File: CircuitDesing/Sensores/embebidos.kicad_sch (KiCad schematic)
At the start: 15 parts

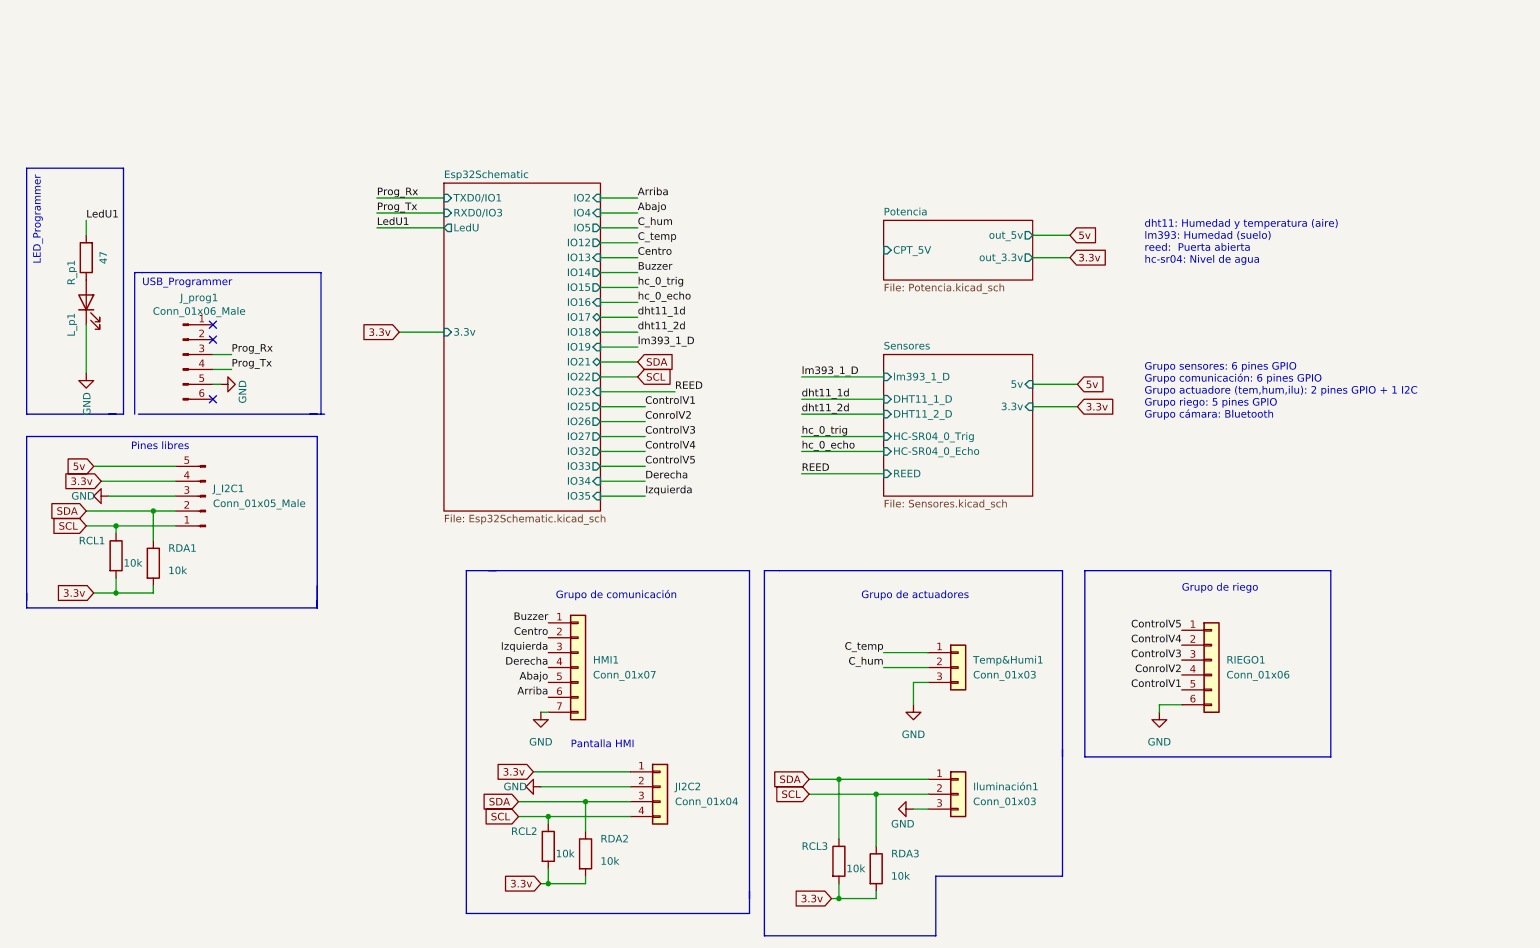
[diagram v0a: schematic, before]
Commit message: Coversores lógicos + alertas + cambios genrales
Coversores lógicos + alertas + cambios generales
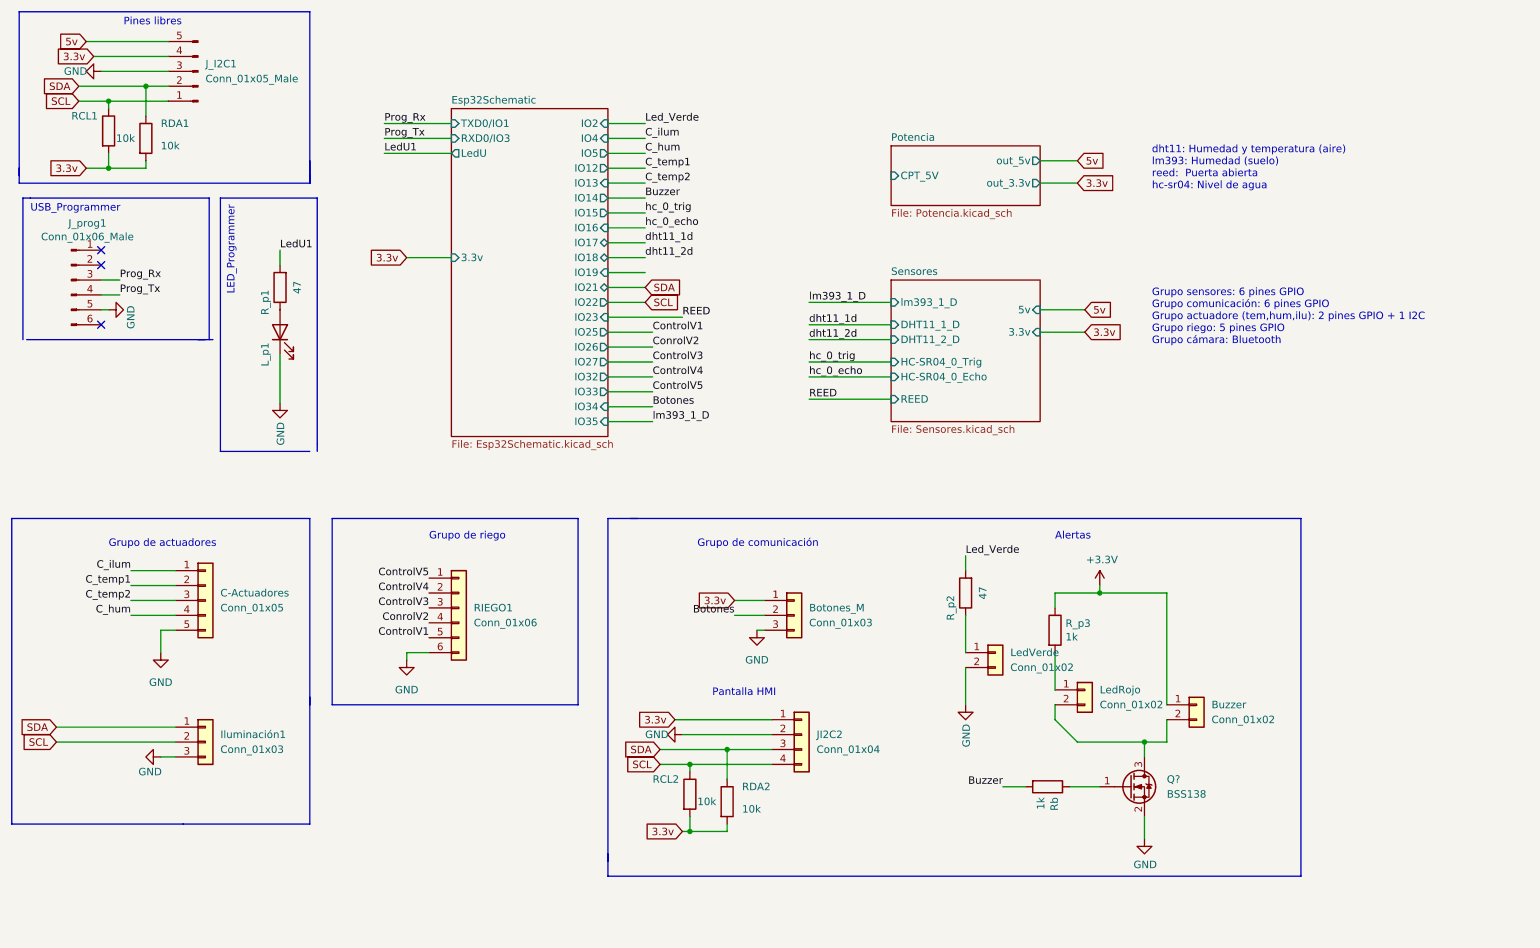
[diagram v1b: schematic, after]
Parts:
- removed HMI1: Conn_01x07, Connector_JST:JST_EH_B7B-EH-A_1x07_P2.50mm_Vertical, symbol Connector_Generic:Conn_01x07
- removed RCL3, RDA3: 10k, Resistor_SMD:R_0805_2012Metric_Pad1.20x1.40mm_HandSolder, symbol Device:R
- removed Temp&Humi1: Conn_01x03, Connector_JST:JST_EH_B3B-EH-A_1x03_P2.50mm_Vertical, symbol Connector_Generic:Conn_01x03
- added Botones_M: Conn_01x03, Connector_JST:JST_EH_B3B-EH-A_1x03_P2.50mm_Vertical, symbol Connector_Generic:Conn_01x03
- added Buzzer, LedRojo, LedVerde: Conn_01x02, symbol Connector_Generic:Conn_01x02
- added C-Actuadores: Conn_01x05, symbol Connector_Generic:Conn_01x05
- added Q?: BSS138, Package_TO_SOT_SMD:SOT-23, symbol Transistor_FET:BSS138
- added R_p2: 47, Resistor_SMD:R_0805_2012Metric_Pad1.20x1.40mm_HandSolder, symbol Device:R
- added R_p3: 1k, symbol Device:R
- added Rb: 1k, Resistor_SMD:R_0603_1608Metric_Pad0.98x0.95mm_HandSolder, symbol Device:R
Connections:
- net 3.3v: now also Botones_M.1 (Pin_1)
- net Buzzer: now also Rb.2
- net C_hum: now also C-Actuadores.4 (Pin_4)
- net GND: now also Botones_M.3 (Pin_3), C-Actuadores.5 (Pin_5), LedVerde.2 (Pin_2), Q?.2 (S)
- new net: LedRojo.1 (Pin_1), R_p3.2
- new net: LedVerde.1 (Pin_1), R_p2.1
- new net: Buzzer.2 (Pin_2), LedRojo.2 (Pin_2), Q?.3 (D)
- new net: Q?.1 (G), Rb.1
- new net +3V3: Buzzer.1 (Pin_1), R_p3.1
- new net Botones: Botones_M.2 (Pin_2)
- new net C_ilum: C-Actuadores.1 (Pin_1)
- new net C_temp1: C-Actuadores.2 (Pin_2)
- new net C_temp2: C-Actuadores.3 (Pin_3)
- new net Led_Verde: R_p2.2
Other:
- note added: "Alertas"
- moved on the sheet: Iluminación1, JI2C2, J_I2C1, J_prog1, L_p1, RCL1, RCL2, RDA1, RDA2, RIEGO1, R_p1
